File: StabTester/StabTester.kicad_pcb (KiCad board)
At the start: 2 copper layers, 20 parts

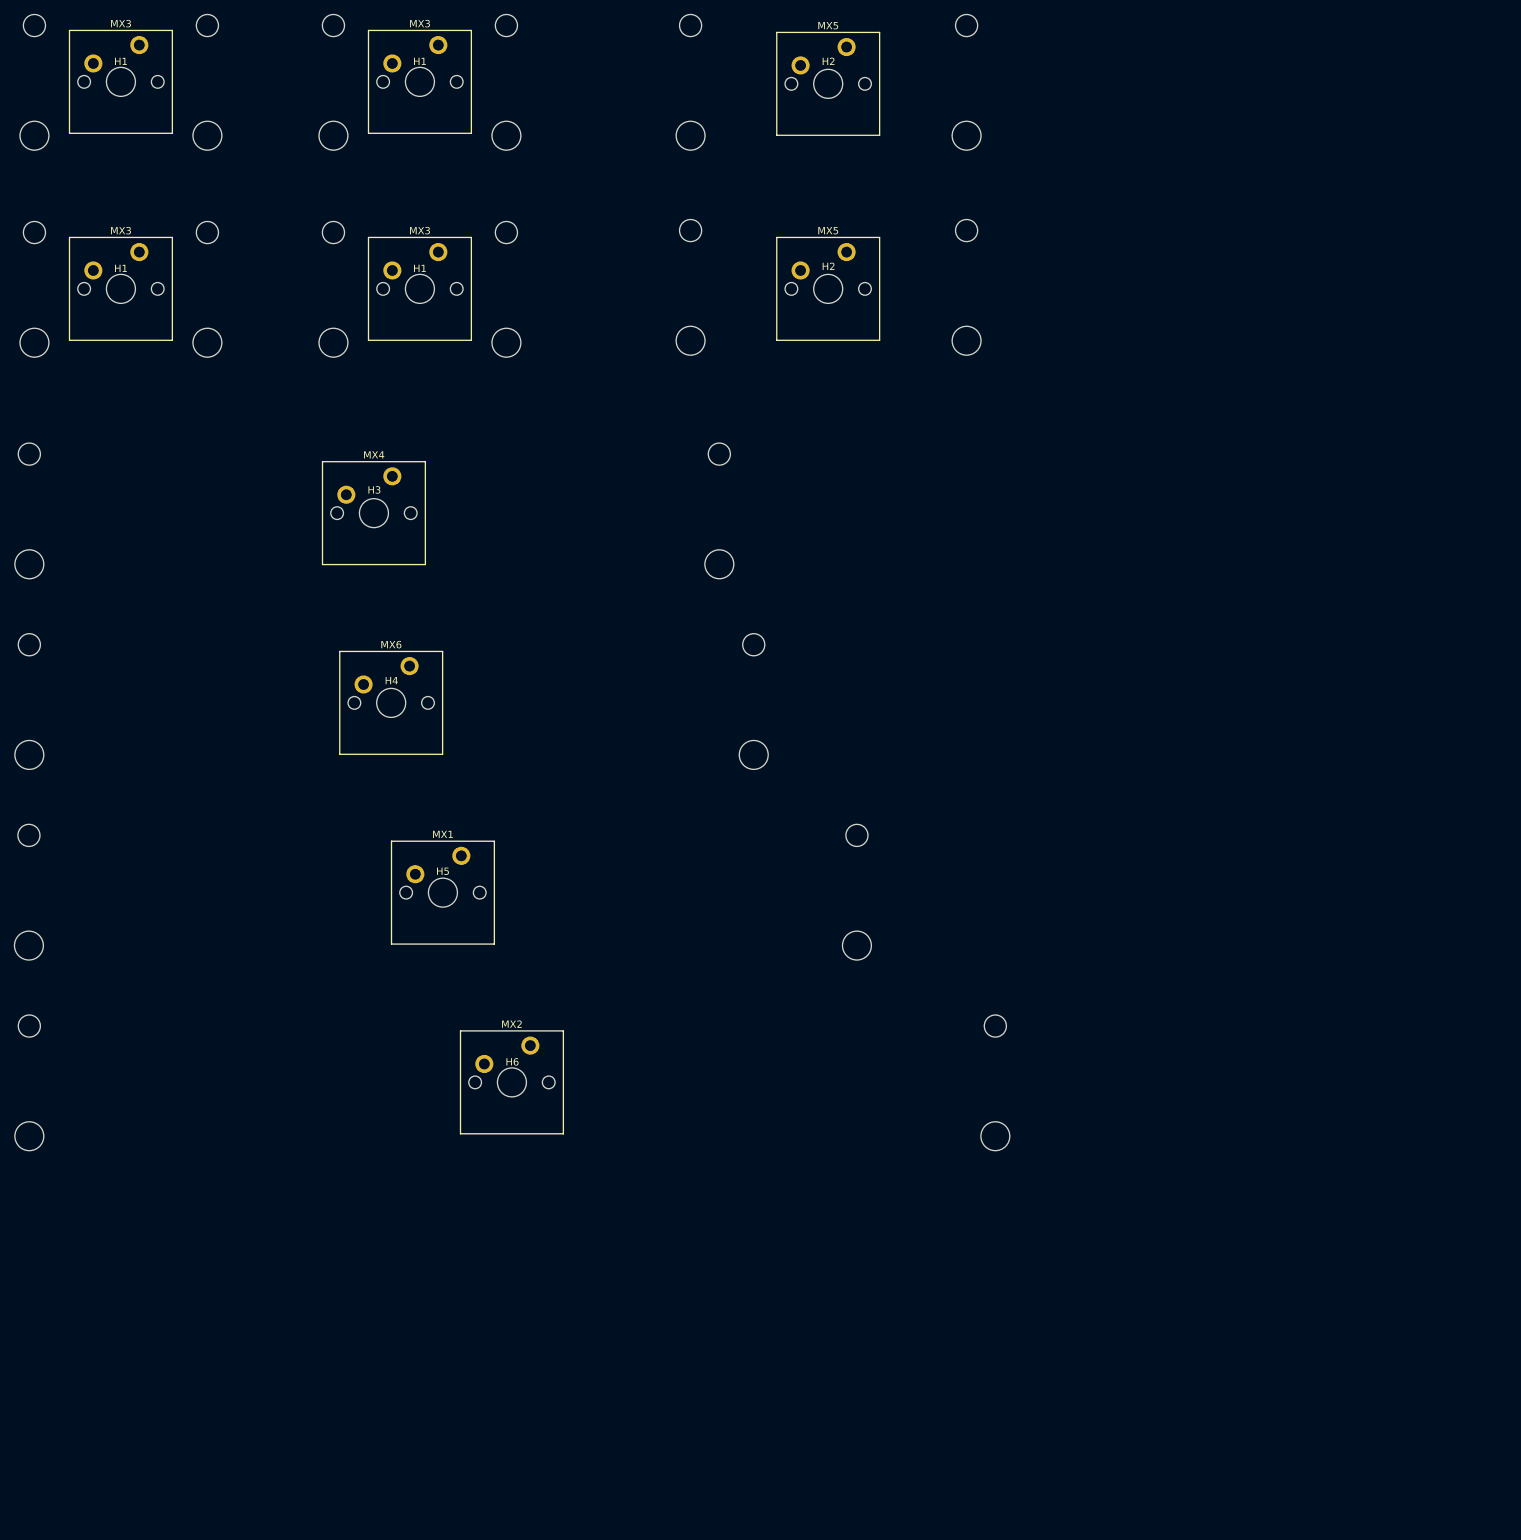
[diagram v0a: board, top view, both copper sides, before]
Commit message: added cosmetics
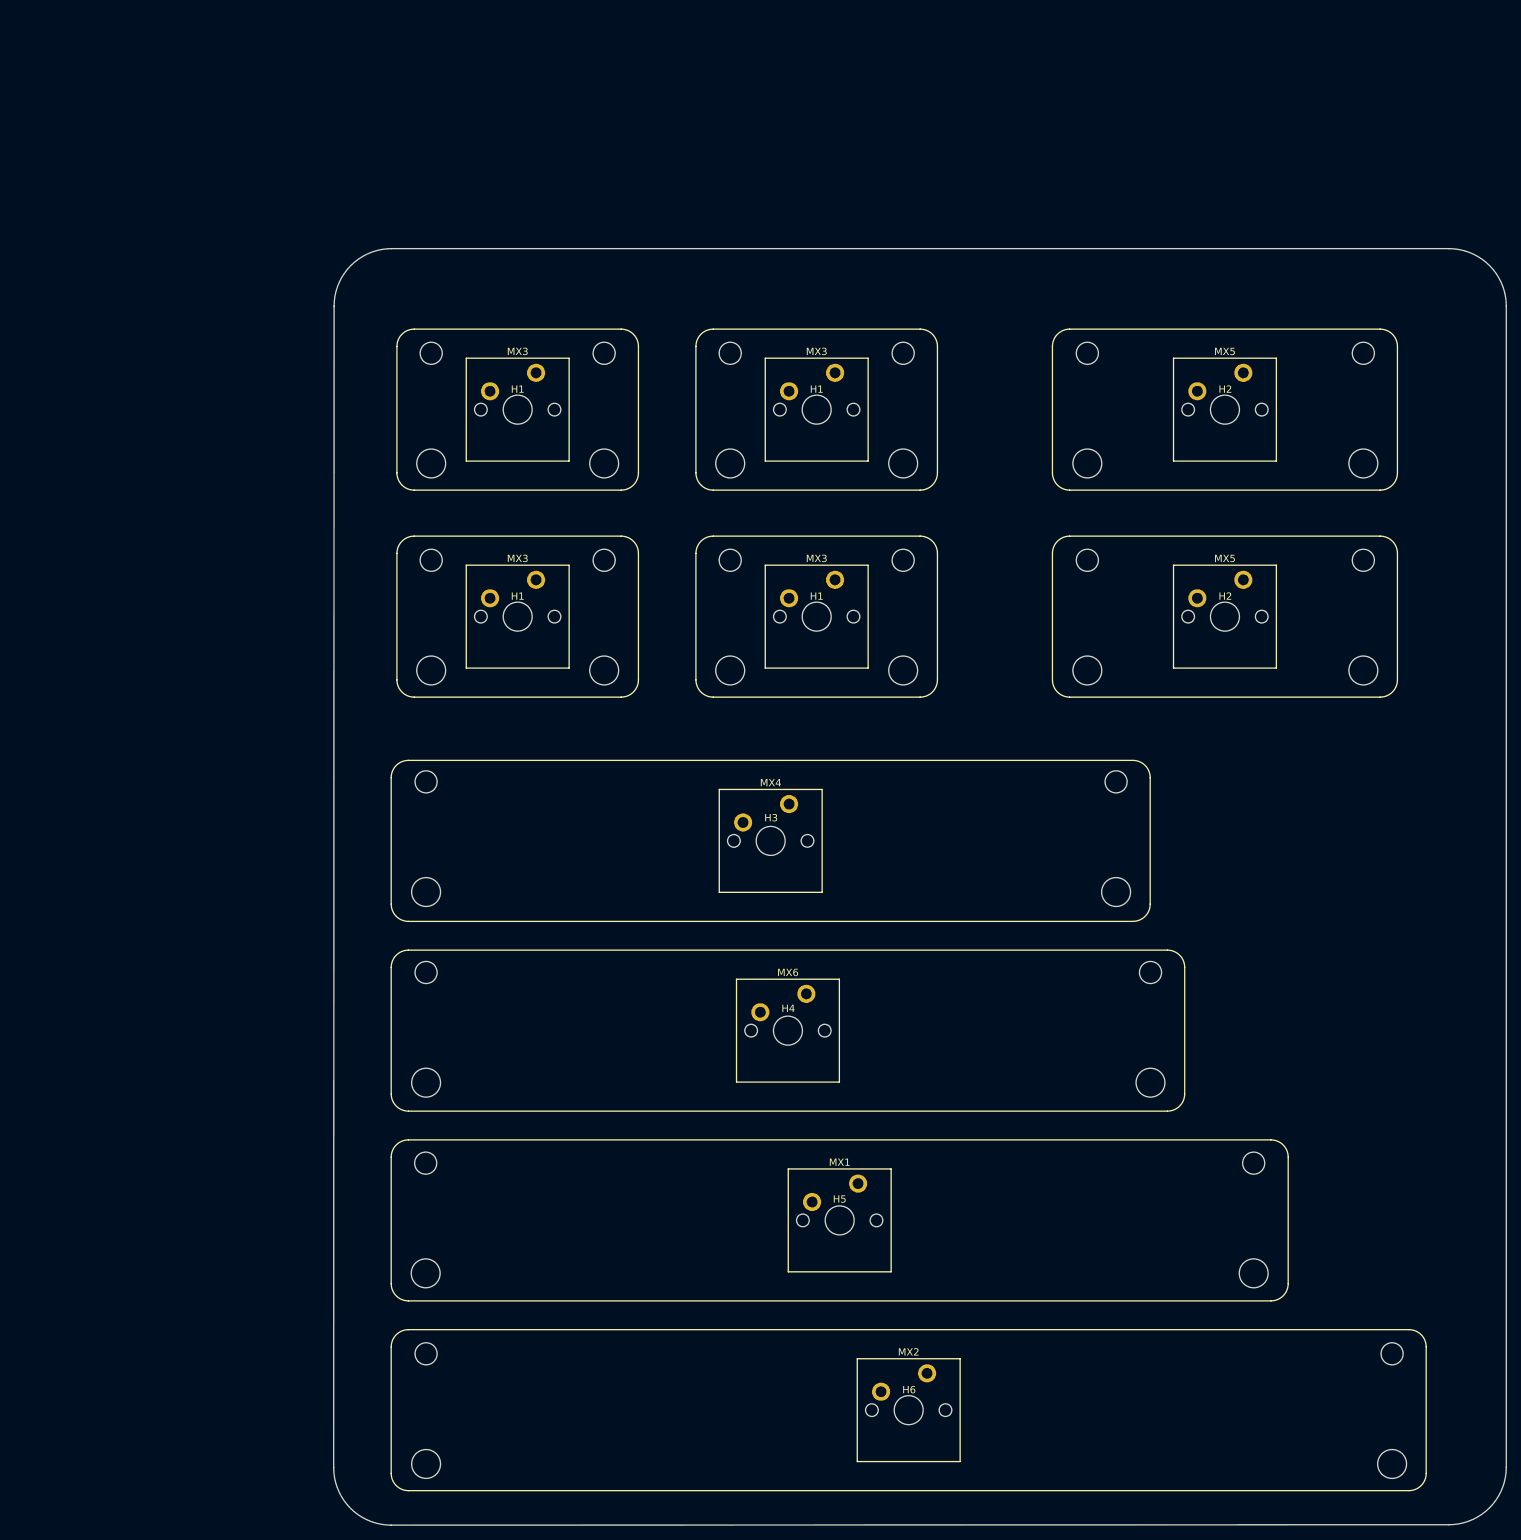
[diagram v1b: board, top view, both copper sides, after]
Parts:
- moved H2 71.2 mm to (208.8, 97.6)
- moved H1 71.0 mm to (152.4, 69.1)
- moved H2 71.0 mm to (208.8, 69.1)
- moved MX3 71.0 mm to (152.4, 98.4)
- moved H1 71.0 mm to (152.4, 97.6)
- moved H6 71.0 mm to (165.2, 207.2)
- moved MX3 71.0 mm to (152.4, 69.8)
- moved MX4 71.0 mm to (146.1, 129.4)
- moved MX6 71.0 mm to (148.4, 155.6)
- moved H1 71.0 mm to (111.1, 97.6)
- moved H1 71.0 mm to (111.1, 69.1)
- moved H3 71.0 mm to (146.1, 128.2)
- moved H4 71.0 mm to (148.5, 154.5)
- moved H5 71.0 mm to (155.6, 180.9)
- moved MX1 71.0 mm to (155.6, 181.8)
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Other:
- board outline added: 161.9 x 176.2 mm
